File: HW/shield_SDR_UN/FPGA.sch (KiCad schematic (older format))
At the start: 68 parts, among them J1 Conn_02x09_Odd_Even, J2 Conn_02x08_Odd_Even, U4 XC6SLX9-2TQG144C, X2 ASE-xxxMHz

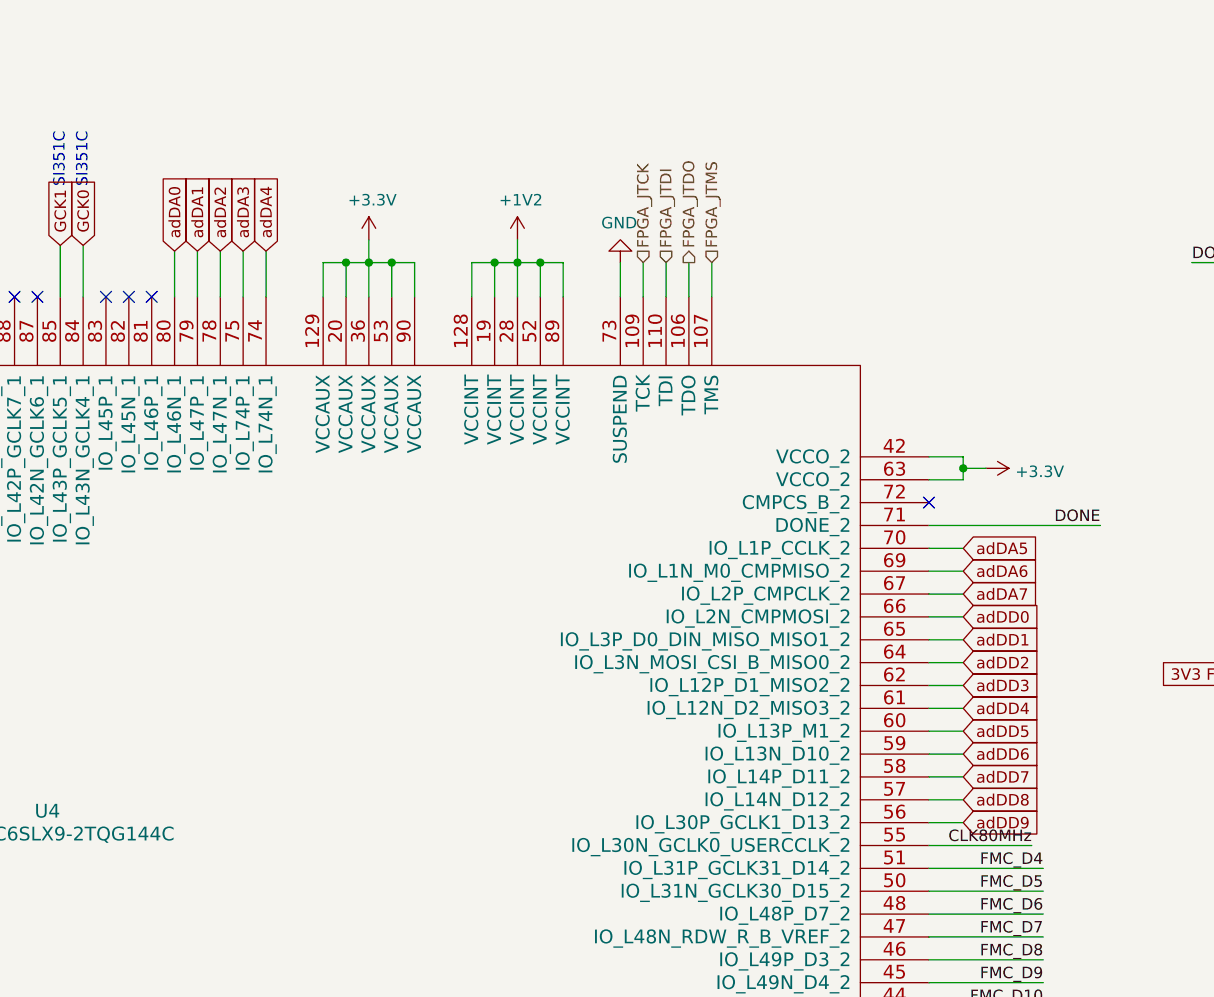
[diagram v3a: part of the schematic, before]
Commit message: organizacion PCB_V4
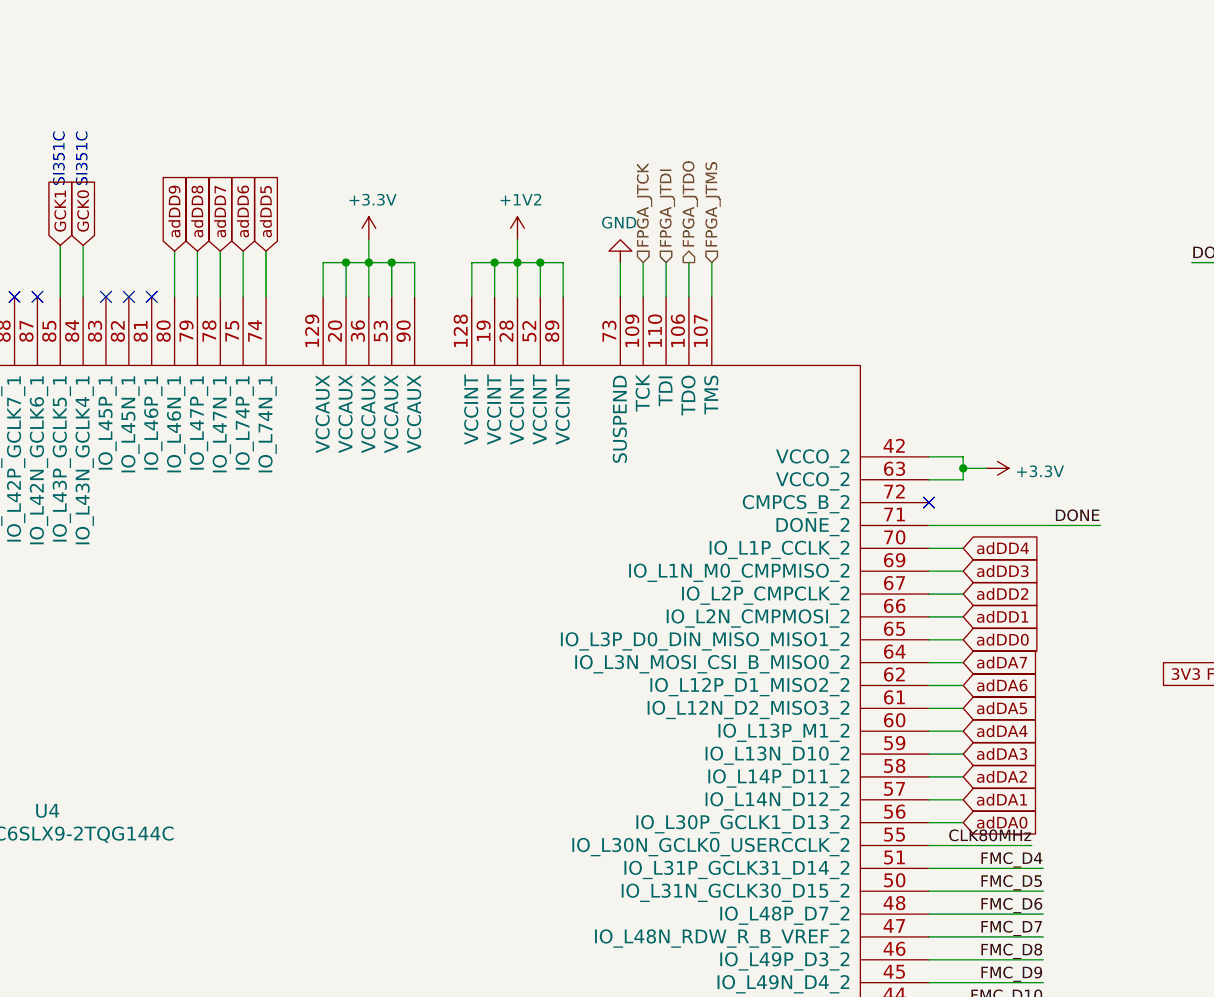
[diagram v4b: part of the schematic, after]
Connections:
- net adDA0: now also U4.56 (IO_L30P_GCLK1_D13_2); no longer U4.80 (IO_L46N_1)
- net adDA1: now also U4.57 (IO_L14N_D12_2); no longer U4.79 (IO_L47P_1)
- net adDA2: now also U4.58 (IO_L14P_D11_2); no longer U4.78 (IO_L47N_1)
- net adDA3: now also U4.59 (IO_L13N_D10_2); no longer U4.75 (IO_L74P_1)
- net adDA4: now also U4.60 (IO_L13P_M1_2); no longer U4.74 (IO_L74N_1)
- net adDA5: now also U4.61 (IO_L12N_D2_MISO3_2); no longer U4.70 (IO_L1P_CCLK_2)
- net adDA6: now also U4.62 (IO_L12P_D1_MISO2_2); no longer U4.69 (IO_L1N_M0_CMPMISO_2)
- net adDA7: now also U4.64 (IO_L3N_MOSI_CSI_B_MISO0_2); no longer U4.67 (IO_L2P_CMPCLK_2)
- net adDD0: now also U4.65 (IO_L3P_D0_DIN_MISO_MISO1_2); no longer U4.66 (IO_L2N_CMPMOSI_2)
- net adDD1: now also U4.66 (IO_L2N_CMPMOSI_2); no longer U4.65 (IO_L3P_D0_DIN_MISO_MISO1_2)
- net adDD2: now also U4.67 (IO_L2P_CMPCLK_2); no longer U4.64 (IO_L3N_MOSI_CSI_B_MISO0_2)
- net adDD3: now also U4.69 (IO_L1N_M0_CMPMISO_2); no longer U4.62 (IO_L12P_D1_MISO2_2)
- net adDD4: now also U4.70 (IO_L1P_CCLK_2); no longer U4.61 (IO_L12N_D2_MISO3_2)
- net adDD5: now also U4.74 (IO_L74N_1); no longer U4.60 (IO_L13P_M1_2)
- net adDD6: now also U4.75 (IO_L74P_1); no longer U4.59 (IO_L13N_D10_2)
- net adDD7: now also U4.78 (IO_L47N_1); no longer U4.58 (IO_L14P_D11_2)
- net adDD8: now also U4.79 (IO_L47P_1); no longer U4.57 (IO_L14N_D12_2)
- net adDD9: now also U4.80 (IO_L46N_1); no longer U4.56 (IO_L30P_GCLK1_D13_2)
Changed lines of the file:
@@
 Wire Wire Line
 	12350 3200 12200 3200
-Text GLabel 8900 1900 1    50   Input ~ 0
+Text GLabel 12350 4400 2    50   Input ~ 0
 adDA0
-Text GLabel 9000 1900 1    50   Input ~ 0
+Text GLabel 12350 4300 2    50   Input ~ 0
 adDA1
-Text GLabel 9100 1900 1    50   Input ~ 0
+Text GLabel 12350 4200 2    50   Input ~ 0
 adDA2
 Text Label 6500 7225 1    50   ~ 0
@@
 Wire Wire Line
 	12200 5600 12675 5600
+Text GLabel 12350 3900 2    50   Input ~ 0
+adDA5
+Text GLabel 12350 3800 2    50   Input ~ 0
+adDA6
+Text GLabel 12350 3700 2    50   Input ~ 0
+adDA7
+Text GLabel 12350 3600 2    50   Input ~ 0
+adDD0
+Text GLabel 12350 3500 2    50   Input ~ 0
+adDD1
+Text GLabel 12350 3400 2    50   Input ~ 0
+adDD2
+Text GLabel 12350 3300 2    50   Input ~ 0
+adDD3
 Text GLabel 12350 3200 2    50   Input ~ 0
-adDA5
-Text GLabel 12350 3300 2    50   Input ~ 0
-adDA6
-Text GLabel 12350 3400 2    50   Input ~ 0
-adDA7
-Text GLabel 12350 3500 2    50   Input ~ 0
-adDD0
-Text GLabel 12350 3600 2    50   Input ~ 0
-adDD1
-Text GLabel 12350 3700 2    50   Input ~ 0
-adDD2
-Text GLabel 12350 3800 2    50   Input ~ 0
-adDD3
-Text GLabel 12350 3900 2    50   Input ~ 0
 adDD4
+Text GLabel 9300 1900 1    50   Input ~ 0
+adDD5
+Text GLabel 9200 1900 1    50   Input ~ 0
+adDD6
+Text GLabel 9100 1900 1    50   Input ~ 0
+adDD7
+Text GLabel 9000 1900 1    50   Input ~ 0
+adDD8
+Text GLabel 8900 1900 1    50   Input ~ 0
+adDD9
+Text GLabel 12350 4100 2    50   Input ~ 0
+adDA3
 Text GLabel 12350 4000 2    50   Input ~ 0
-adDD5
-Text GLabel 12350 4100 2    50   Input ~ 0
-adDD6
-Text GLabel 12350 4200 2    50   Input ~ 0
-adDD7
-Text GLabel 12350 4300 2    50   Input ~ 0
-adDD8
-Text GLabel 12350 4400 2    50   Input ~ 0
-adDD9
-Text GLabel 9200 1900 1    50   Input ~ 0
-adDA3
-Text GLabel 9300 1900 1    50   Input ~ 0
 adDA4
 Wire Wire Line
